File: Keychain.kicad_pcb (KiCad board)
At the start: 4 copper layers, 53 x 47 mm, 61 parts, among them J1 Micro_SD_Card, J2 Conn_01x04, J3 USB_A, U1 IMX6UL_BGA289, U2 DDR3_BGA96, U3 AZ1117C-3.3, U4 AZ1117C-1.5, Y1 Crystal_GND24

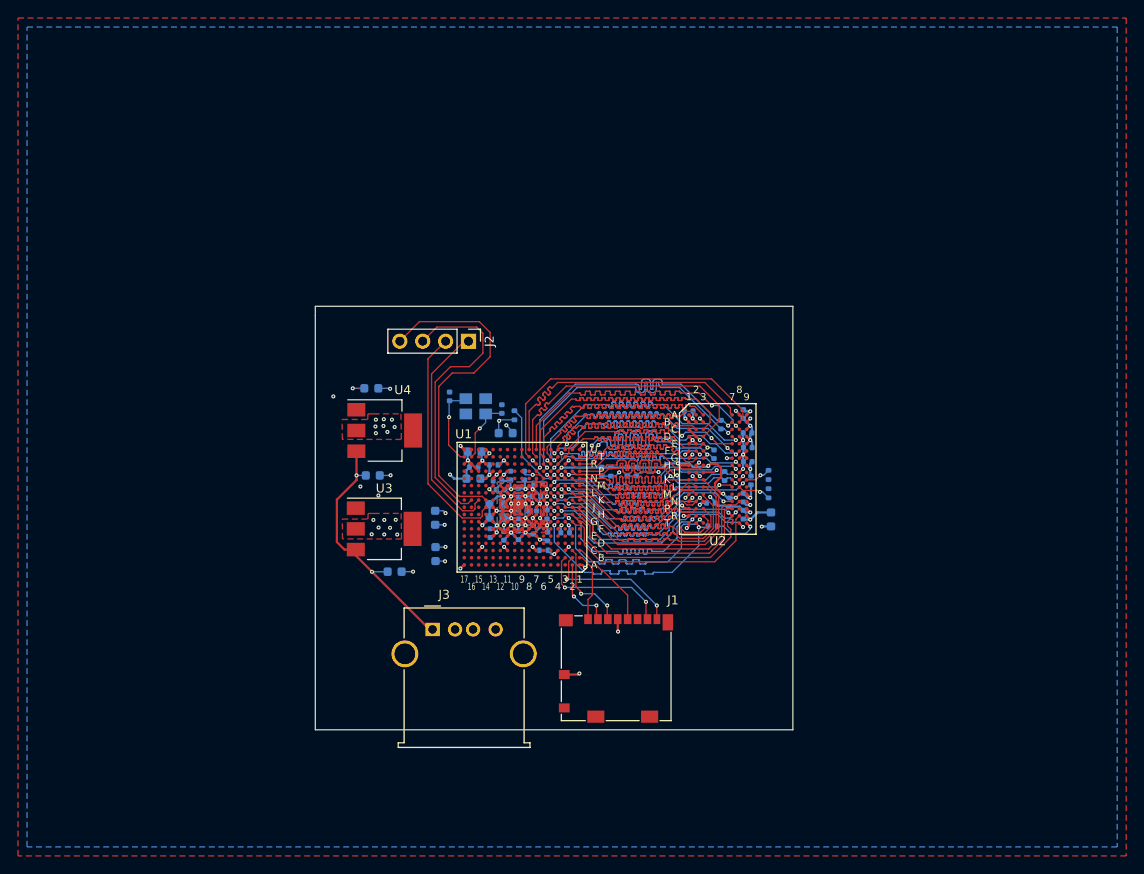
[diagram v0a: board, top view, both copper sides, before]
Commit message: New layout!
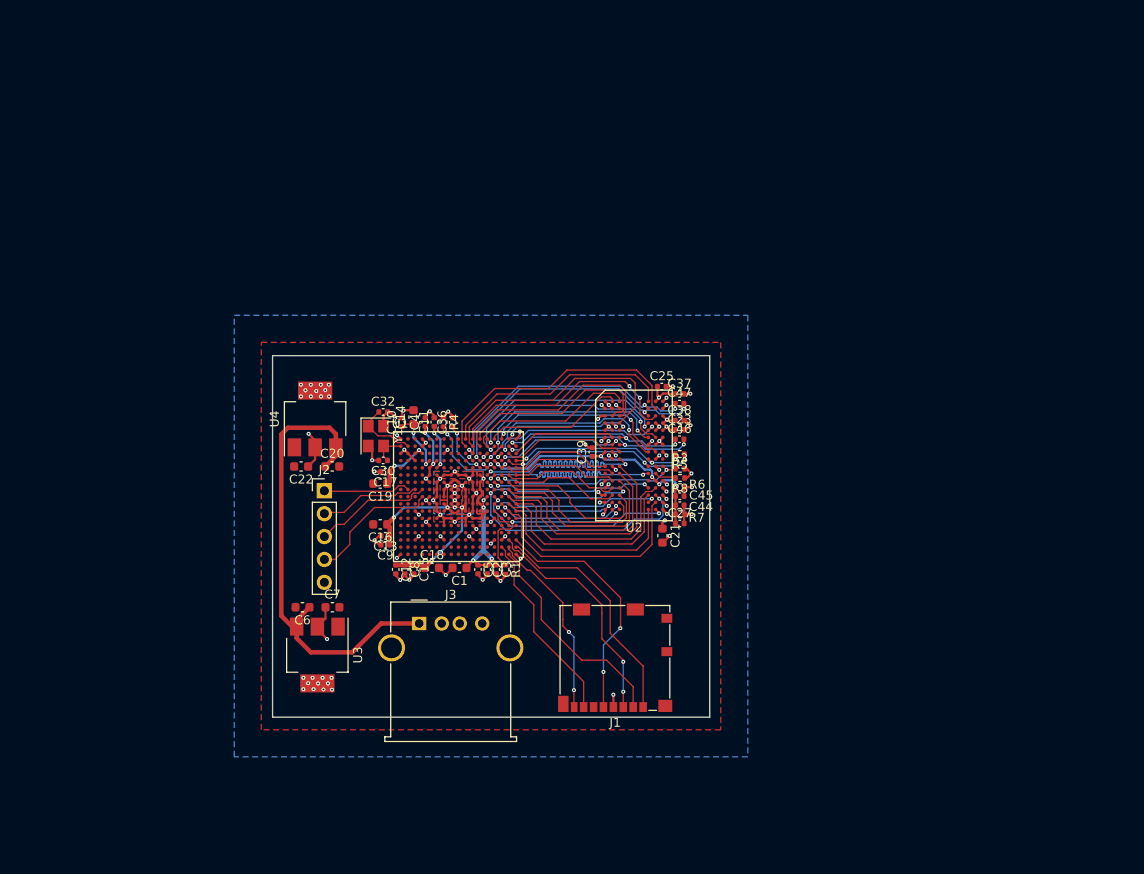
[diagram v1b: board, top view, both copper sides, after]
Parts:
- removed C24: 10uF, Capacitor_SMD:C_0603_1608Metric
- removed C26, C28, C29, C31, C33, C35, C51, C52, C53, C54: 0.22uF, Capacitor_SMD:C_0402_1005Metric
- C1, C10, C11, C12, C13, C14, C15, C16, C17, C18, C19, C2, C20, C21, C22, C23, C25, C27, C3, C30, C32, C36, C37, C38, C39, C4, C44, C45, C46, C47, C5, C6, C7, C8, C9, R1, R3, R4, R5, R6, R7, R8, Y1: moved to F.Cu
- J2: footprint Connector_PinHeader_2.54mm:PinHeader_1x04_P2.54mm_Vertical -> Connector_PinHeader_2.54mm:PinHeader_1x05_P2.54mm_Vertical
- moved R1 23.5 mm to (145.1, 92.2), turned to 270 degrees
- moved J2 23.1 mm to (125.0, 83.5), turned to 0 degrees
- moved C8 16.7 mm to (133.9, 92.2), turned to 270 degrees
- moved C39 16.2 mm to (154.8, 79.2), turned to 90 degrees
- moved U3 15.8 mm to (124.2, 101.7), turned to 270 degrees
- moved C25 15.3 mm to (162.4, 71.9), turned to 0 degrees
- moved C7 15.1 mm to (125.9, 96.4), turned to 0 degrees
- moved C9 14.8 mm to (131.8, 89.5), turned to 180 degrees
- moved C12 14.6 mm to (132.9, 92.2), turned to 270 degrees
- moved C15 14.0 mm to (134.9, 92.2)
- moved C32 13.2 mm to (131.5, 74.7), turned to 0 degrees
- moved C13 13.2 mm to (131.8, 88.5), turned to 180 degrees
- moved C16 12.9 mm to (131.2, 87.2)
- moved C21 12.2 mm to (162.5, 88.5)
- moved C22 11.7 mm to (122.4, 80.8), turned to 180 degrees
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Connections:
- net /DDR/A0 renamed /A0
- net /DDR/A1 renamed /A1
- net /DDR/A10 renamed /A10
- net /DDR/A11 renamed /A11
- net /DDR/A12 renamed /A12
- net /DDR/A13 renamed /A13
- net /DDR/A14 renamed /A14
- net /DDR/A2 renamed /A2
- net /DDR/A3 renamed /A3
- net /DDR/A4 renamed /A4
- net /DDR/A5 renamed /A5
- net /DDR/A6 renamed /A6
- net /DDR/A7 renamed /A7
- net /DDR/A8 renamed /A8
- net /DDR/A9 renamed /A9
- net /DDR/BA0 renamed /BA0
- net /DDR/BA1 renamed /BA1
- net /DDR/BA2 renamed /BA2
- net /DDR/CAS# renamed /CAS#
- net /DDR/CK+ renamed /CK+
- net /DDR/CK- renamed /CK-
- net /DDR/CKE0 renamed /CKE0
- net /DDR/CS0# renamed /CS0#
- net /DDR/DML renamed /DML
- net /DDR/DMU renamed /DMU
- net /DDR/DQL0 renamed /DQL0
- net /DDR/DQL2 renamed /DQL2
- net /DDR/DQL3 renamed /DQL3
- net /DDR/DQL4 renamed /DQL4
- net /DDR/DQL5 renamed /DQL5
- net /DDR/DQSL+ renamed /DQSL+
- net /DDR/DQSL- renamed /DQSL-
- net /DDR/DQSU+ renamed /DQSU+
- net /DDR/DQSU- renamed /DQSU-
- net /DDR/DQU0 renamed /DQU0
- net /DDR/DQU2 renamed /DQU2
- net /DDR/DQU6 renamed /DQU6
- net /DDR/ODT0 renamed /ODT0
- net /DDR/RAS# renamed /RAS#
- net /DDR/RESET# renamed /RESET#
- net /DDR/WE# renamed /WE#
- net /DDR/ZQ renamed /ZQ
- net /DDR/ZQPAD renamed /ZQPAD
- net ARM_CAP renamed /ARM_CAP
- net HIGH_CAP renamed /HIGH_CAP
- net NVCC_PLL renamed /NVCC_PLL
- net Net-(C30-Pad1) renamed /XTALO
- net Net-(C32-Pad1) renamed /XTALI
- net SD_CLK renamed /SD_CLK
- net SD_CMD renamed /SD_CMD
- net SD_D0 renamed /SD_D0
- net SD_D1 renamed /SD_D1
- net SD_D2 renamed /SD_D2
- net SD_D3 renamed /SD_D3
- net SNVS_CAP renamed /SNVS_CAP
- net SOC_CAP renamed /SOC_CAP
- net VDD_HIGH_CAP renamed /VDD_HIGH_CAP
- C1 pad 1: +3V3 -> +1V5
- C2 pad 1: +3V3 -> +1V5
- C27 pad 1: +1V5 -> VREFDDR
- C3 pad 1: +3V3 -> +1V5
- C4 pad 1: +1V5 -> +3V3
- C5 pad 1: +3V3 -> +1V5
- J2 pad 1: Net-(J2-Pad1) -> /RX
- J2 pad 2: Net-(J2-Pad2) -> /CTS
- J2 pad 3: Net-(J2-Pad3) -> /TX
- J2 pad 4: Net-(J2-Pad4) -> /RTS
- U1 pad H10: +3V3 -> +1V5
- U1 pad H9: +3V3 -> +1V5
- U1 pad J10: +3V3 -> +1V5
- U1 pad J14: Net-(J2-Pad2) -> /RTS
- U1 pad J9: +3V3 -> +1V5
- U1 pad K10: +3V3 -> +1V5
- U1 pad K14: Net-(J2-Pad4) -> /TX
- U1 pad K15: Net-(J2-Pad1) -> /CTS
- U1 pad K16: Net-(J2-Pad3) -> /RX
- U1 pad K9: +3V3 -> +1V5
- U1 pad N13: +1V5 -> +3V3
- U1 pad P12: +1V5 -> +3V3
- U1 pad P3: /DDR/DQU5 -> /DQU5
- U1 pad P5: /DDR/DQU4 -> /DQU4
- U1 pad R1: /DDR/DQU7 -> /DQU7
- U1 pad R4: /DDR/DQU3 -> /DQU3
- U1 pad T5: /DDR/DQL6 -> /DQL6
- U1 pad U3: /DDR/DQU1 -> /DQU1
- U1 pad U4: /DDR/DQL7 -> /DQL7
- U1 pad U6: /DDR/DQL1 -> /DQL1
- U2 pad A2: /DDR/DQL6 -> /DQL7
- U2 pad A3: /DDR/DQL1 -> /DQL6
- U2 pad C2: /DDR/DQL7 -> /DQL1
- U2 pad F2: /DDR/DQU3 -> /DQU7
- U2 pad F7: /DDR/DQU1 -> /DQU3
- U2 pad G2: /DDR/DQU7 -> /DQU5
- U2 pad H7: /DDR/DQU5 -> /DQU4
- U2 pad H8: /DDR/DQU4 -> /DQU1
- U3 pad 1: GND -> Net-(U3-Pad1)
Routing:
- net GND: track 122.7 -> 84.0 mm, vias 62 -> 63
- net Net-(J2-Pad4): track 37.4 -> 0.00 mm
- net /DDR/DQL6: track 33.5 -> 0.00 mm
- net /DDR/DQL1: track 32.9 -> 0.00 mm
- net Net-(J2-Pad3): track 32.4 -> 0.00 mm
- net /DDR/DQU1: track 31.9 -> 0.00 mm, vias 2 -> 0
- net /DDR/DQL7: track 31.8 -> 0.00 mm
- net Net-(J2-Pad2): track 25.5 -> 0.00 mm
- net /DDR/DQU4: track 25.1 -> 0.00 mm, vias 2 -> 0
- net /DDR/DQU5: track 25.1 -> 0.00 mm, vias 2 -> 0
- net Net-(J2-Pad1): track 24.8 -> 0.00 mm
- net /DDR/DQU3: track 24.3 -> 0.00 mm, vias 2 -> 0
- net +5V: track 28.8 -> 52.7 mm, vias 2 -> 0
- net /DDR/DQU7: track 23.7 -> 0.00 mm
- net /DQU4: track 0.00 -> 22.5 mm, vias 0 -> 2
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- added copper zone on In2.Cu, net +1V5
- added copper zone on In2.Cu, net +3V3
- added copper zone on In1.Cu, net GND
- removed copper zone on PWR, net +1V5
- removed copper zone on B.Cu, net +3V3
- removed copper zone on F.Cu, net +3V3
- removed copper zone on PWR, net +3V3
- removed copper zone on B.Cu, net /ARM_CAP
- removed copper zone on B.Cu, net /SOC_CAP
- removed copper zone on GND, net GND
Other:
- board size 53 x 47 mm -> 48.5 x 40.1 mm
- net class DDR added: clearance 0.127, trace_width 0.145, via_dia 0.45, via_drill 0.2
- net class Default: trace_width 0.127 -> 0.1
- net class POWER added: clearance 0.127, trace_width 0.25, via_dia 0.45, via_drill 0.2
- rule pad_to_mask_clearance: 0 -> 0.05
- rule trace_min: 0.127 -> 0.1
